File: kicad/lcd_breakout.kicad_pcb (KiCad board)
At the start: 2 copper layers, 4 parts, among them J1 Conn_01x05_Male, U1 AY0438X-P, U2 DE119

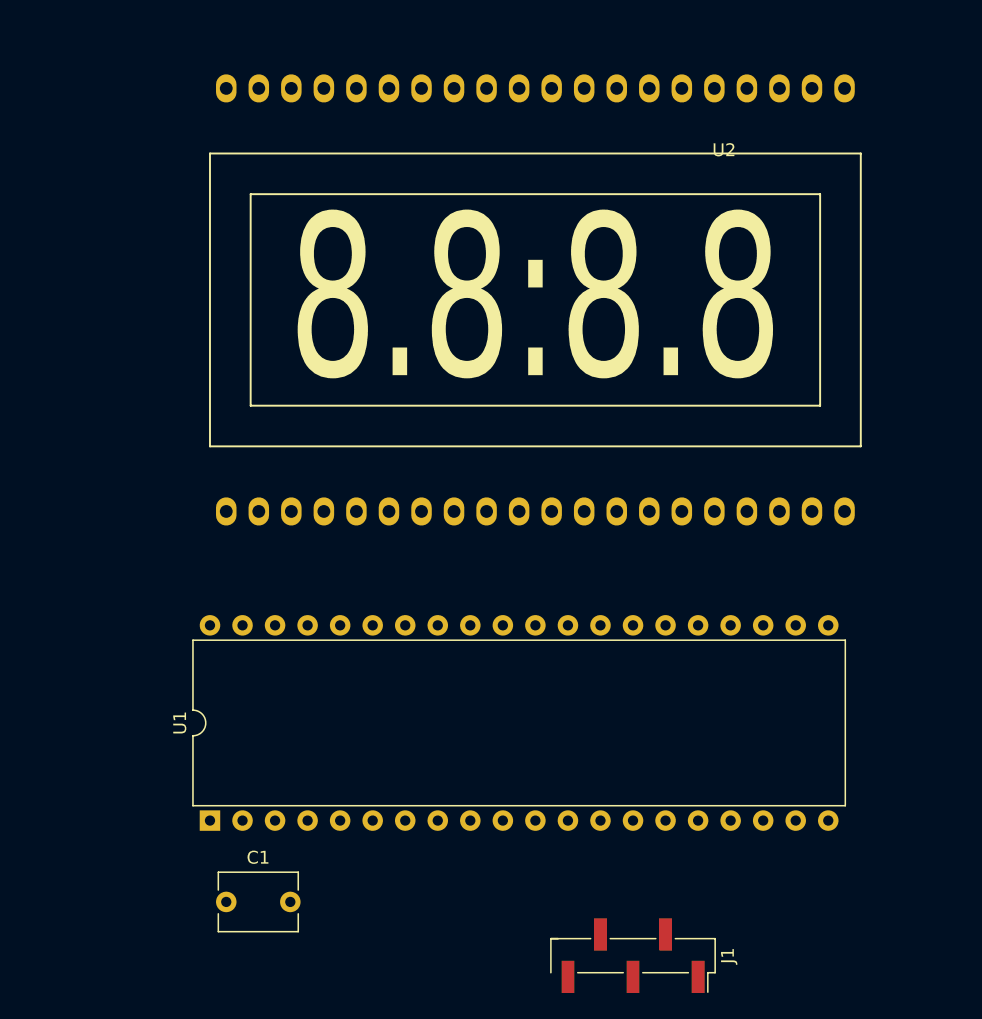
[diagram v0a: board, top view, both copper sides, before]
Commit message: Work on routing
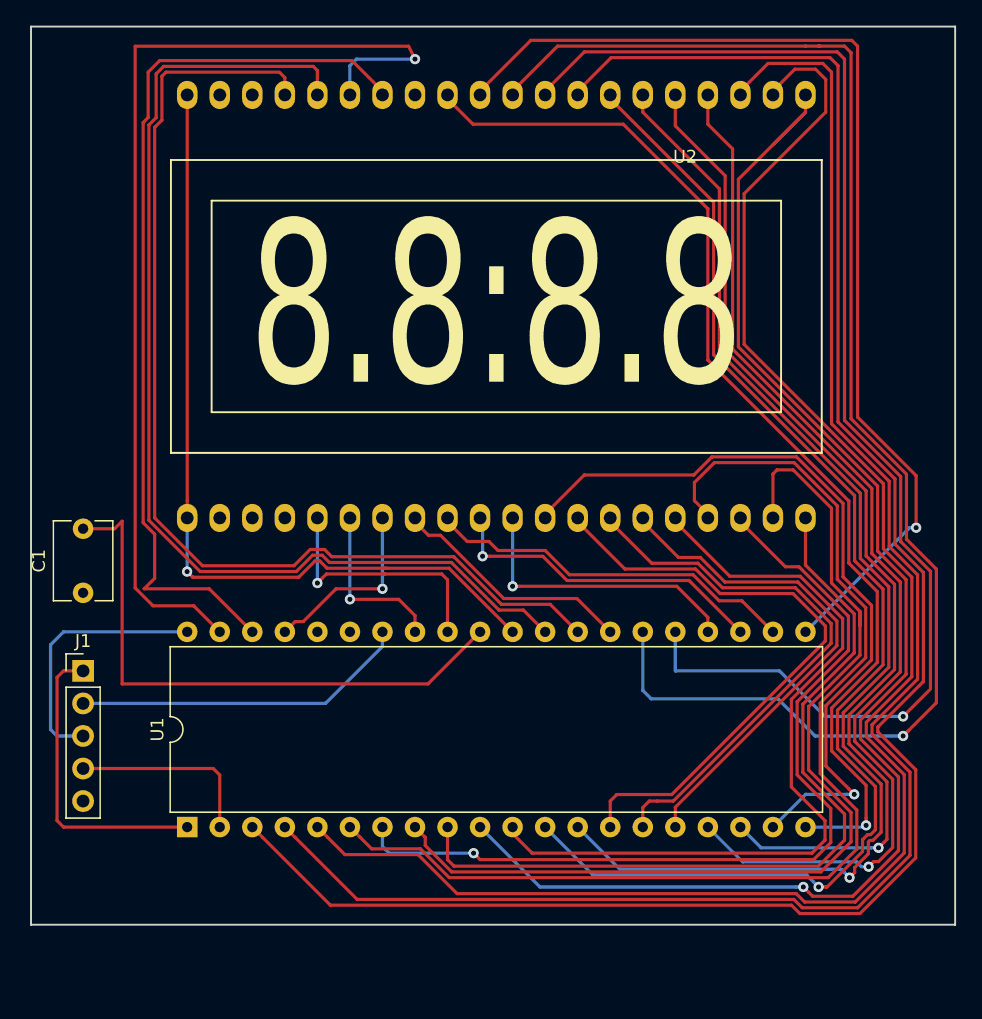
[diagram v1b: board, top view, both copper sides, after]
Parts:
- J1: footprint Connector_PinHeader_2.54mm:PinHeader_1x05_P2.54mm_Vertical_SMD_Pin1Right -> Connector_PinHeader_2.54mm:PinHeader_1x05_P2.54mm_Vertical
- moved J1 48.3 mm to (100.6, 110.2), turned to 0 degrees
- moved C1 26.6 mm to (100.6, 104.1), turned to 90 degrees
- moved U2 3.09 mm to (132.8, 81.8)
- moved U1 1.85 mm to (108.7, 122.4)
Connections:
- net VCC renamed VDD
- C1 pad 1: Net-(C1-Pad1) -> GND
- C1 pad 2: GND -> Net-(C1-Pad2)
- U1 pad 31: Net-(C1-Pad1) -> Net-(C1-Pad2)
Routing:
- net Net-(U1-Pad3): track 0.00 -> 145.6 mm
- net Net-(U1-Pad4): track 0.00 -> 128.3 mm
- net Net-(U1-Pad5): track 0.00 -> 126.4 mm
- net Net-(U1-Pad26): track 0.00 -> 112.1 mm, vias 0 -> 1
- net Net-(U1-Pad10): track 0.00 -> 109.5 mm, vias 0 -> 1
- net Net-(U1-Pad25): track 0.00 -> 102.3 mm, vias 0 -> 1
- net Net-(U1-Pad12): track 0.00 -> 99.0 mm, vias 0 -> 1
- net Net-(U1-Pad13): track 0.00 -> 95.8 mm, vias 0 -> 1
- net Net-(U1-Pad6): track 0.00 -> 88.9 mm
- net Net-(U1-Pad29): track 0.00 -> 85.5 mm
- net Net-(U1-Pad20): track 0.00 -> 85.4 mm, vias 0 -> 1
- net Net-(U1-Pad17): track 0.00 -> 84.5 mm, vias 0 -> 1
- net Net-(U1-Pad28): track 0.00 -> 83.9 mm
- net Net-(U1-Pad21): track 0.00 -> 83.1 mm, vias 0 -> 1
- net Net-(U1-Pad39): track 0.00 -> 80.7 mm, vias 0 -> 1
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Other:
- board outline added: 72.1 x 70.1 mm
